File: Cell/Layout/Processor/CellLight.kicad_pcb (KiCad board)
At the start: 2 copper layers, 100 x 16 mm, 30 parts, among them J1 Conn_01x05, J2 Conn_01x02, J3 Conn_01x02, J4 Conn_01x02, J5 Conn_01x03, J6 Conn_01x03, SW1 SW_Push, U1 STM32G030F6P6, U10 74LVC1G125, U11 LM1085-5.0, U2 74LVC1G125, U3 MB85RC256, U4 74LVC1G125, U5 AP2112K-3.3, U6 SN74LVC1T45DBVR, U7 74LVC1G125, U8 74LVC1G125, U9 74LVC1G125

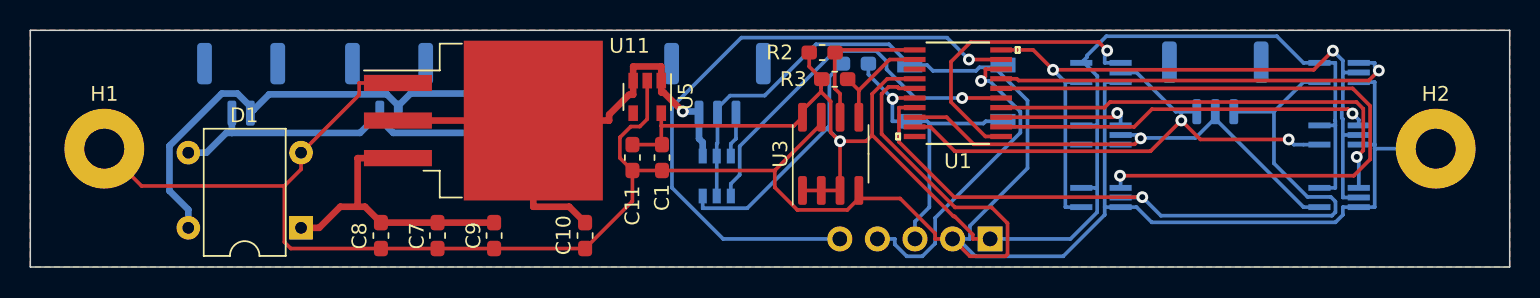
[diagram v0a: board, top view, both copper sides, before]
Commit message: Do the processor board layout
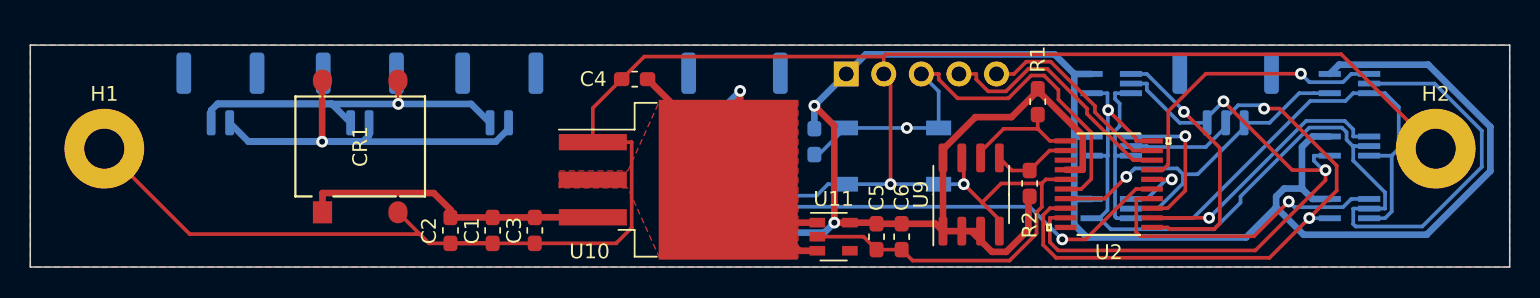
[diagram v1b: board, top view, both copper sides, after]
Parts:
- removed D1: DF02M, Diode_THT:Diode_Bridge_DIP-4_W7.62mm_P5.08mm
- removed the U5 at (149.4, 130.2)
- added CR1: DF01S, df01s:DF01S, F.Cu at (130.0, 133.6)
- added U11: AP2112K-3.3, Package_TO_SOT_SMD:SOT-23-5, F.Cu at (162.0, 139.7)
- moved J4 21.4 mm to (120.5, 130.0)
- moved J2 17.5 mm to (139.4, 130.0)
- moved C5 17.3 mm to (164.9, 139.7)
- moved C6 17.1 mm to (166.6, 139.7)
- moved R1 14.9 mm to (175.8, 130.5), turned to 270 degrees
- moved R2 14.9 mm to (175.2, 136.1), turned to 90 degrees
- moved J1 14.8 mm to (162.8, 128.7), turned to 270 degrees
- moved U10 13.8 mm to (151.5, 135.8)
- moved U2 11.9 mm to (180.6, 136.1)
- moved C4 11.1 mm to (148.6, 129.0), turned to 180 degrees
- moved U9 9.89 mm to (171.3, 136.8)
- moved SW1 6.08 mm to (165.9, 134.2), turned to 0 degrees
- moved R3 5.96 mm to (160.7, 133.2), turned to 270 degrees
- moved C2 4.71 mm to (136.1, 139.2)
- moved C1 3.74 mm to (138.9, 139.2)
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- renumbered C7 to C1, C8 to C2, C9 to C3, C10 to C4, C11 to C5, C1 to C6, R2 to R1, R3 to R2, R1 to R3, U6 to U1, U11 to U10, U1 to U2, U2 to U3, U7 to U5, U8 to U6, U9 to U7, U10 to U8, U3 to U9
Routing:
- net CH1_RX_EN: track 47.3 -> 4.65 mm
- net 3.3V: track 116.0 -> 148.4 mm, vias 1 -> 2
- net SWCLK: track 43.0 -> 13.6 mm, vias 1 -> 0
- net CH1_DATA: track 52.6 -> 26.2 mm
- net COM_DATA: track 49.9 -> 67.9 mm, vias 2 -> 1
- net CH2_DATA: track 33.2 -> 46.1 mm, vias 1 -> 2
- net NRST: track 21.9 -> 33.4 mm
- net CH2_TX_EN: track 30.4 -> 20.5 mm
- net GND: track 216.5 -> 225.5 mm, vias 0 -> 2
- net CH1_TX_EN: track 27.6 -> 19.9 mm
- net CH3_DATA: track 36.4 -> 43.9 mm
- net CH3_TX_EN: track 25.3 -> 18.1 mm
- net PRI_LO: track 26.6 -> 31.5 mm, vias 0 -> 1
- net Net-(U1-Pad4): track 25.6 -> 30.3 mm
- net SWDIO: track 21.8 -> 17.1 mm, vias 1 -> 0
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- added copper zone on F.Cu, net 5V
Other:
- board size 100 x 16 mm -> 100 x 15 mm
